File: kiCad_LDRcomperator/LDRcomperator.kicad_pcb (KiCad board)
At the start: 2 copper layers, 50 x 60 mm, 18 parts, among them J1 Screw_Terminal_01x02, J2 Conn_01x02_MountingPin, J3 Conn_01x02_MountingPin

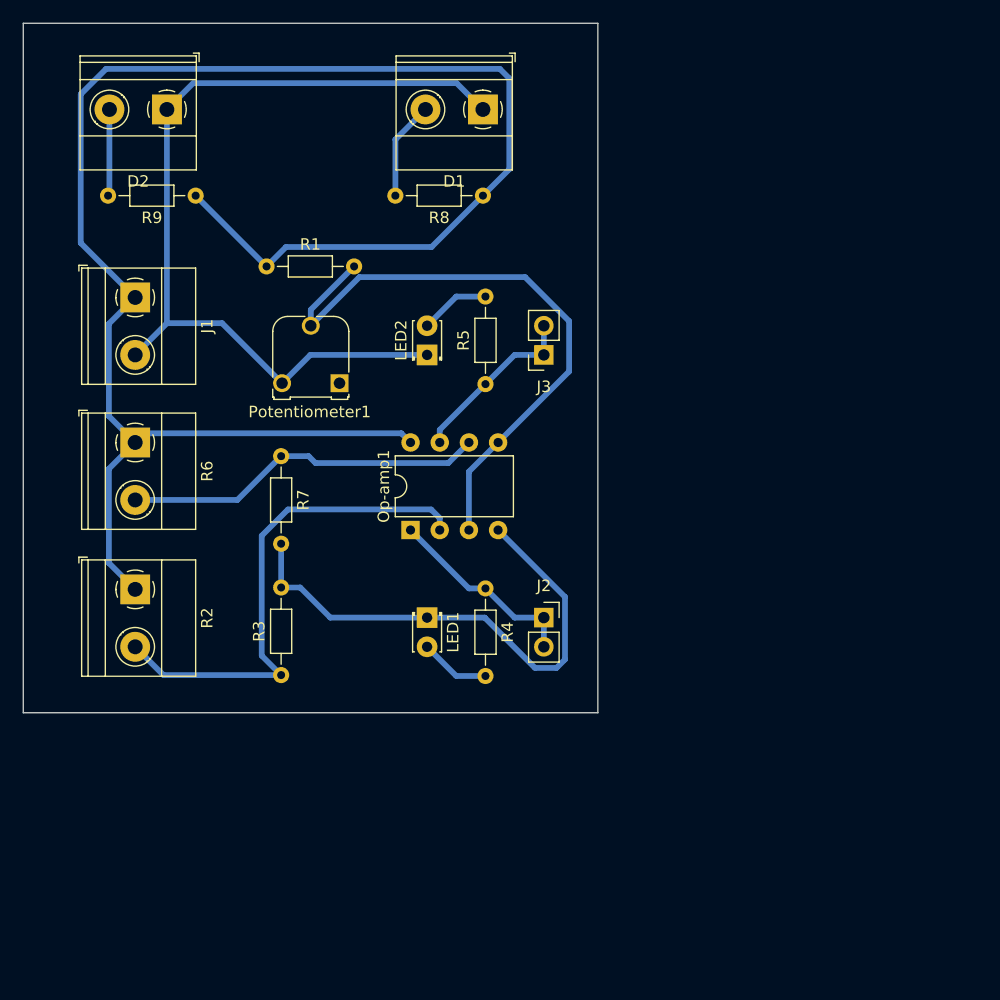
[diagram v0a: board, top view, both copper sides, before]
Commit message: Rapporten
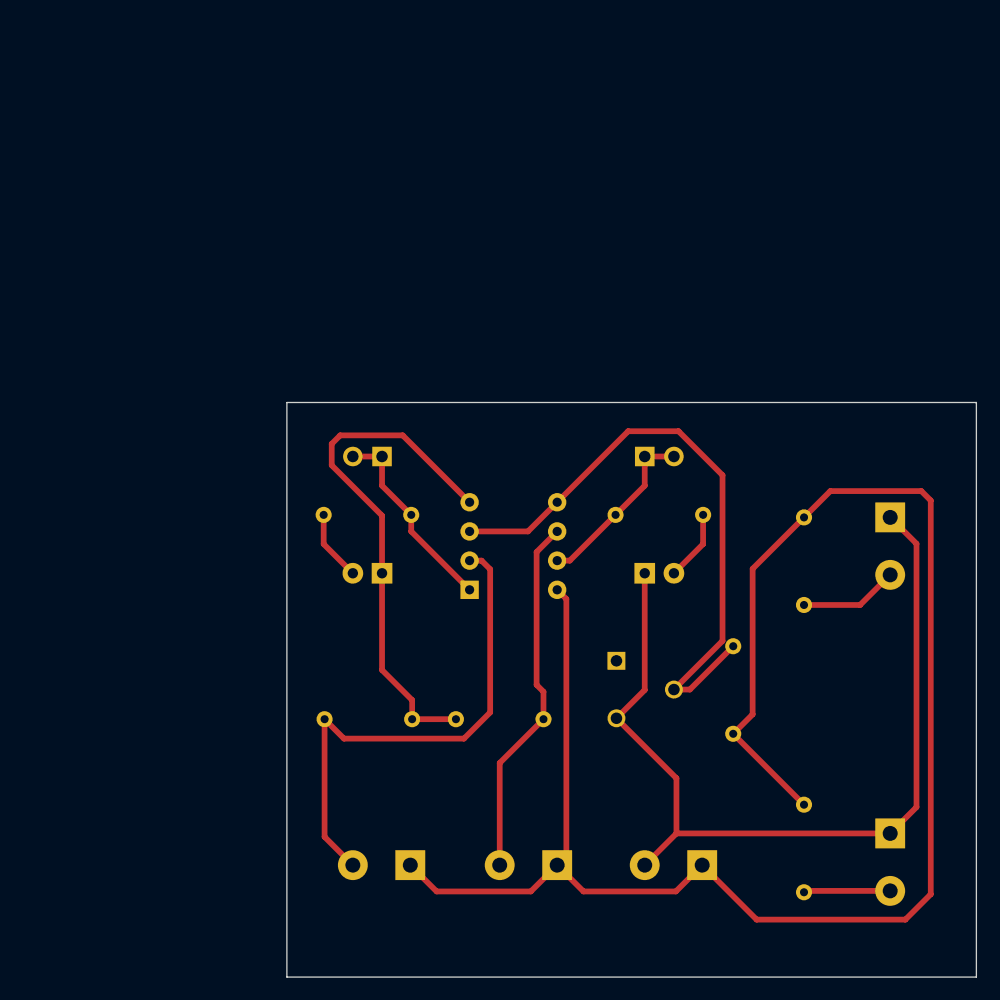
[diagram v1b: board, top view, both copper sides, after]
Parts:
- D1, D2, J1, J2, J3, LED1, LED2, Op-amp1, Potentiometer1, R1, R2, R3, R4, R5, R6, R7, R8, R9: moved to B.Cu
- moved D2 89.1 mm to (207.9, 128.0), turned to -90 degrees
- moved R9 74.9 mm to (200.4, 125.5), turned to -90 degrees
- moved J1 69.8 mm to (191.6, 130.8), turned to 180 degrees
- moved R1 57.5 mm to (194.3, 119.3), turned to 90 degrees
- moved R6 52.0 mm to (179.0, 130.8), turned to 180 degrees
- moved D1 50.2 mm to (207.9, 100.5), turned to -90 degrees
- moved R8 39.6 mm to (200.4, 100.5), turned to -90 degrees
- moved Potentiometer1 34.1 mm to (184.1, 113.0), turned to -90 degrees
- moved R2 33.9 mm to (166.2, 130.8), turned to 180 degrees
- moved R7 32.3 mm to (177.8, 118.1), turned to 180 degrees
- moved LED2 26.8 mm to (186.6, 105.4), turned to 0 degrees
- moved J2 19.9 mm to (163.7, 95.2), turned to 90 degrees
- moved R5 16.1 mm to (184.0, 100.3), turned to 0 degrees
- moved J3 12.5 mm to (186.6, 95.2), turned to -90 degrees
- moved R4 9.09 mm to (166.3, 100.3), turned to 180 degrees
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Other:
- board size 50 x 60 mm -> 60 x 50 mm
